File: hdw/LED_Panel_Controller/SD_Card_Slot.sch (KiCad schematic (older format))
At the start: 1 part

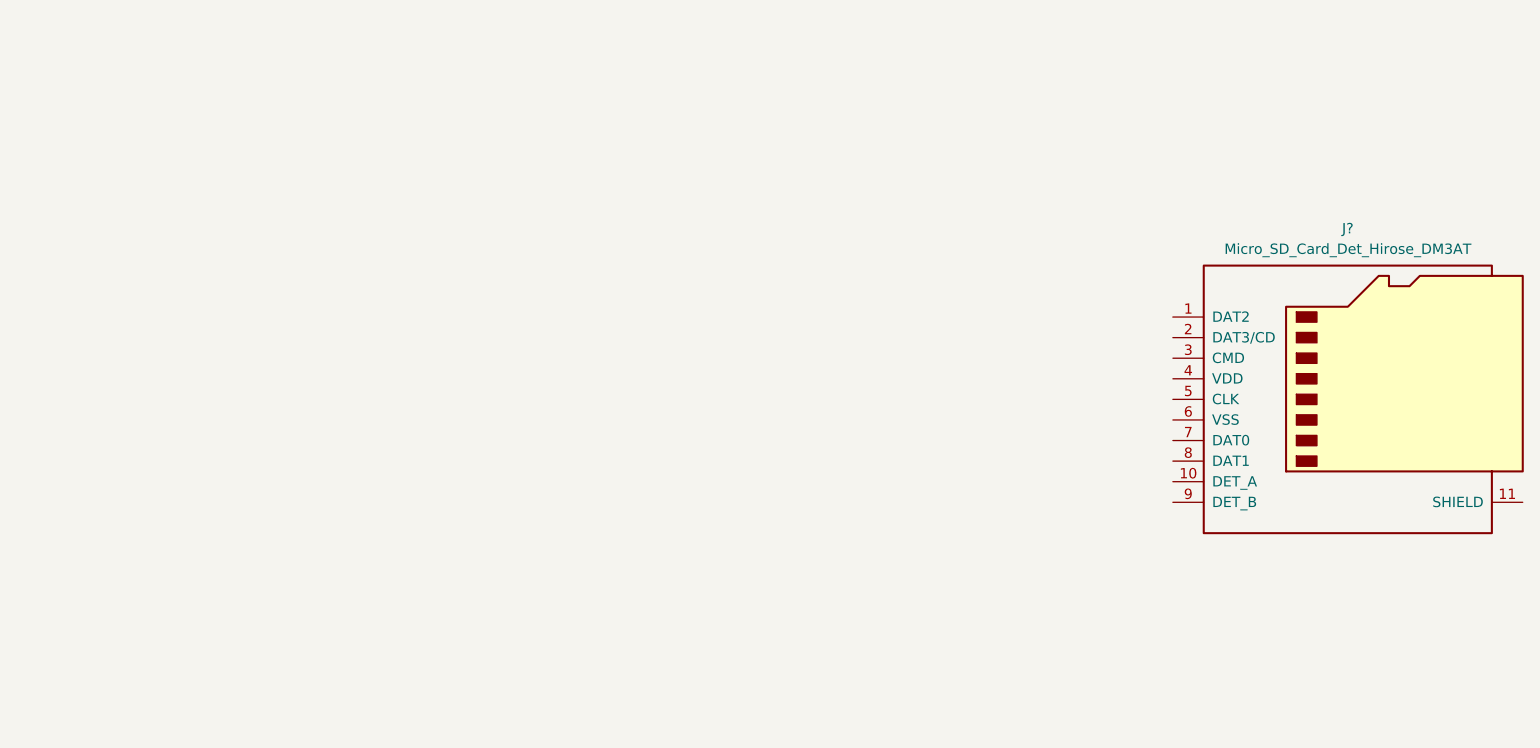
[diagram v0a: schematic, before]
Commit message: log's first
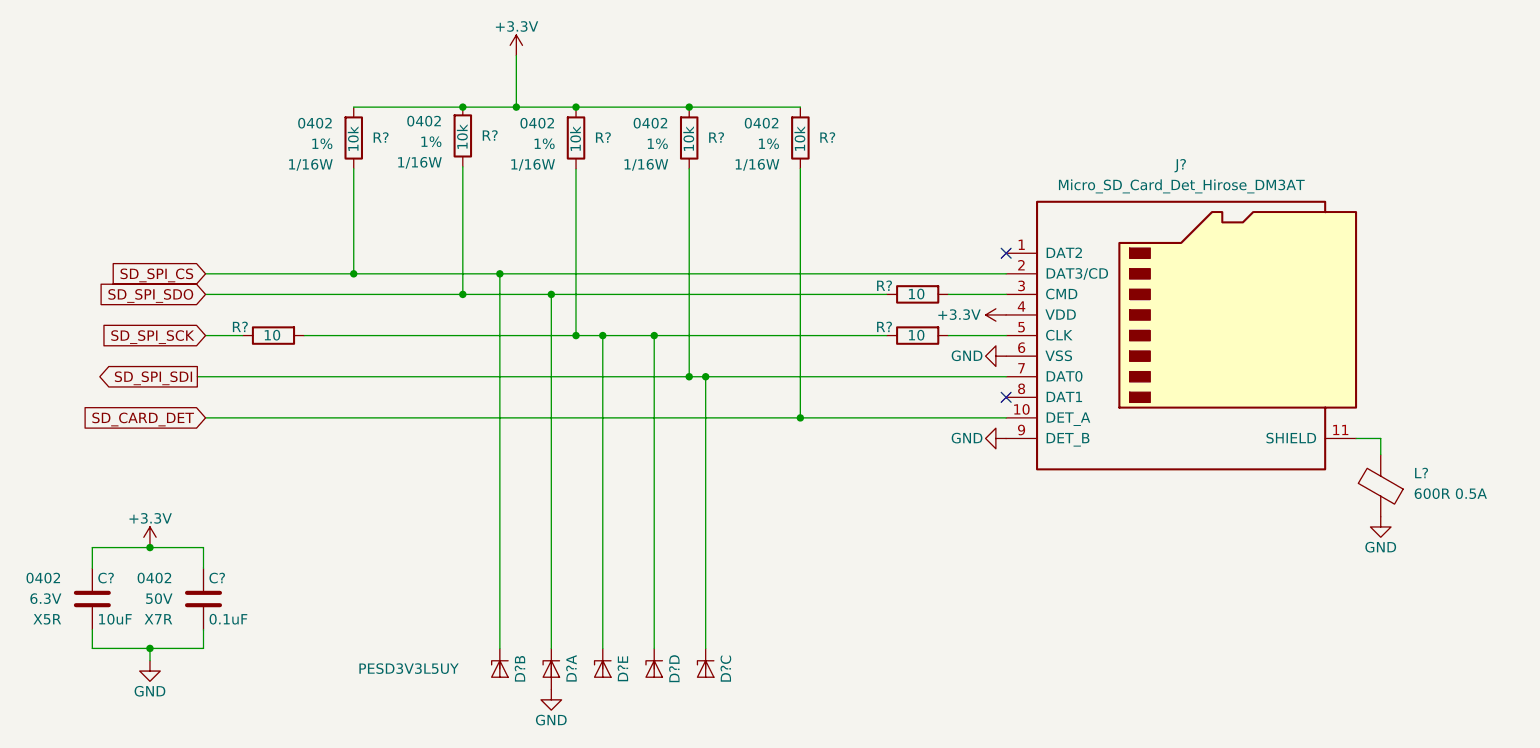
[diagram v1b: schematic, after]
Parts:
- added C?: 0.1uF, Capacitors_SMD:C_0402, symbol Custom_Library:C_Custom
- added C?: 10uF, Capacitors_SMD:C_0402, symbol Custom_Library:C_Custom
- added D? (x5): PESD3V3L5UY, Package_TO_SOT_SMD:SOT-363_SC-70-6, symbol Power_Protection:PESD3V3L5UY
- added L?: 600R 0.5A, Inductors_SMD:L_0402, symbol Device:Ferrite_Bead
- added R? (x5): 10k, Resistors_SMD:R_0402, symbol Custom_Library:R_Custom
- added R? (x3): 10, Resistors_SMD:R_0402, symbol Custom_Library:R_Custom
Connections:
- net SD_CARD_DET: now reaches J?.10 (DET_A)
- net SD_CARD_DET: now also R?.2
- net at J?.11 (SHIELD): now also L?.2
- net SD_SPI_CS: now reaches J?.2 (DAT3/CD)
- net SD_SPI_CS: now also D?.3 (K2), R?.2
- net at J?.3 (CMD): now also R?.1
- net +3V3: now reaches J?.4 (VDD)
- net +3V3: now also C?.1, C?.1, R?.1, R?.1, R?.1, R?.1, R?.1
- net at J?.5 (CLK): now also R?.1
- net GND: now reaches J?.6 (VSS)
- net GND: now also J?.9 (DET_B), C?.2, C?.2, D?.2 (A), L?.1
- net SD_SPI_SDI: now reaches J?.7 (DAT0)
- net SD_SPI_SDI: now also D?.4 (K3), R?.2
- new net: D?.5 (K4), D?.6 (K5), R?.1, R?.2, R?.2
- new net SD_SPI_SCK: R?.2
- new net SD_SPI_SDO: D?.1 (K1), R?.2, R?.2
- no-connect marks 0 -> 2
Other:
- moved on the sheet: J?
